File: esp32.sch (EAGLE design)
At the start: 4 parts, among them U1 ESP32MOD

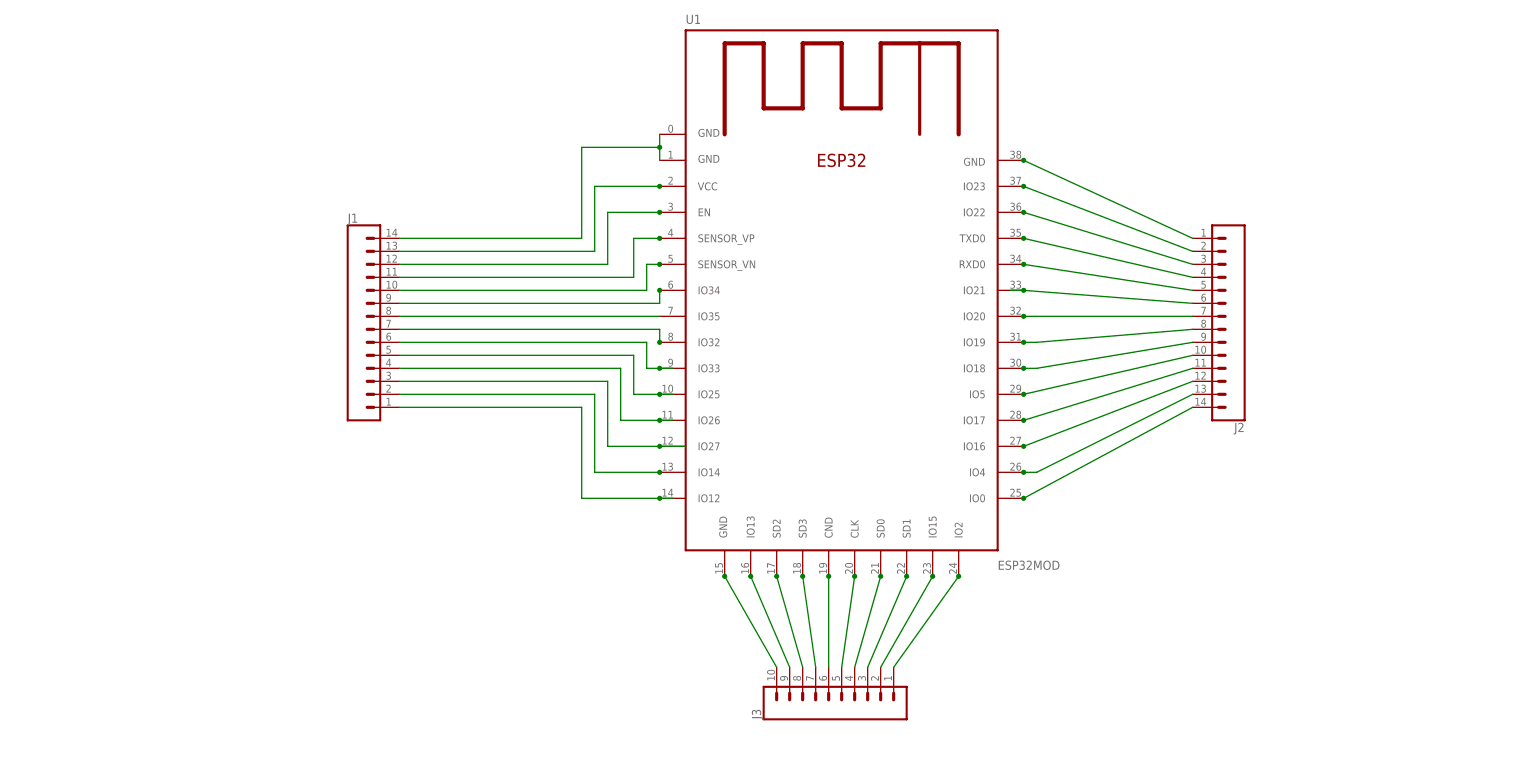
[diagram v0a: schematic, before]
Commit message: connected dual line headers
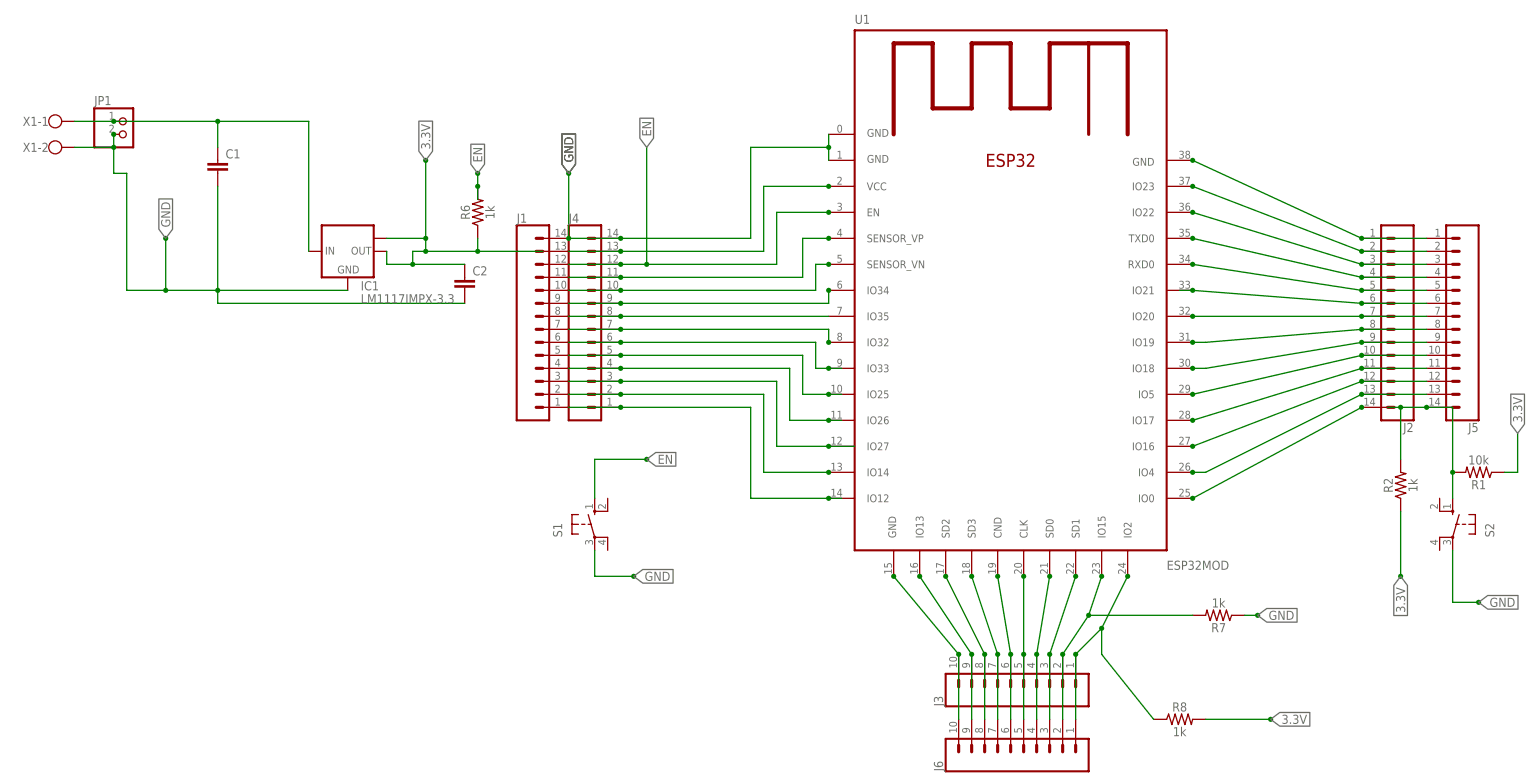
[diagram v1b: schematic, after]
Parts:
- added C1, C2: (no value), rcl:C-EU025-050X050
- added IC1: LM1117IMPX-3.3, lm1117:LM1117IMPX-3.3
- added J4, J5: (no value), SparkFun-Connectors:CONN_14LONGPADS
- added J6: (no value), SparkFun-Connectors:CONN_10"
- added JP1: (no value), pinhead:PINHD-1X2
- added R1: 10k, SparkFun-Resistors:1KOHM-HORIZ-1/4W-1%
- added R2, R6, R7, R8: 1k, SparkFun-Resistors:1KOHM-HORIZ-1/4W-1%
- added S1, S2: (no value), switch-omron:10-XX
- added X1: (no value), con-wago-500:W237-102
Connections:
- new net 3.3V: C2.1, IC1.OUT, IC1.OUT1, R1.1, R2.1, R6.1, R8.2
- new net EN: J1.12, J4.12, R6.2, S1.S, U1.EN
- new net N$21: C1.1, IC1.IN, JP1.1, X1-1.KL
- net GND: now also C1.2, C2.2, IC1.GND, J4.14, J5.1, J6.10, JP1.2, R7.1, S1.P, S2.P, X1-2.KL
- net N$1: now also J5.7
- net N$10: now also J4.5
- net N$11: now also J4.4
- net N$12: now also J4.3
- net N$13: now also J4.2
- net N$14: now also J4.1
- net N$15: now also J5.5
- net N$16: now also J5.4
- net N$17: now also J5.3
- net N$18: now also J5.2
- net N$19: now also J5.10
- net N$2: now also J4.11
- net N$20: now also J5.6
- net N$22: now also J5.8
- net N$23: now also J5.9
- net N$25: now also J5.11
- net N$26: now also J5.12
- net N$27: now also J5.13
- net N$3: now also J4.10
- net N$30: now also J6.9
- net N$31: now also J6.8
- net N$32: now also J6.7
- net N$33: now also J6.6
- net N$34: now also J6.5
- net N$35: now also J6.4
- net N$36: now also J6.3
- net N$37: now also J6.2, R7.2
- net N$38: now also J6.1, R8.1
- net N$4: now also J4.13
- net N$5: now also J5.14, R1.2, R2.2, S2.S; no longer J1.12, U1.EN
- net N$6: now also J4.9
- net N$7: now also J4.8
- net N$8: now also J4.7
- net N$9: now also J4.6
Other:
- moved on the sheet: J1, J2, J3, U1
